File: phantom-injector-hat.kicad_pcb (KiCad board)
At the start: 2 copper layers, 65 x 44.8 mm, 42 parts, among them J1 Conn_02x20_Odd_Even, J2 Conn_02x03_Top_Bottom, J3 Conn_01x03, J4 Conn_01x03, SW1 SW_SPST, U1 LT8362EMSE-PBF

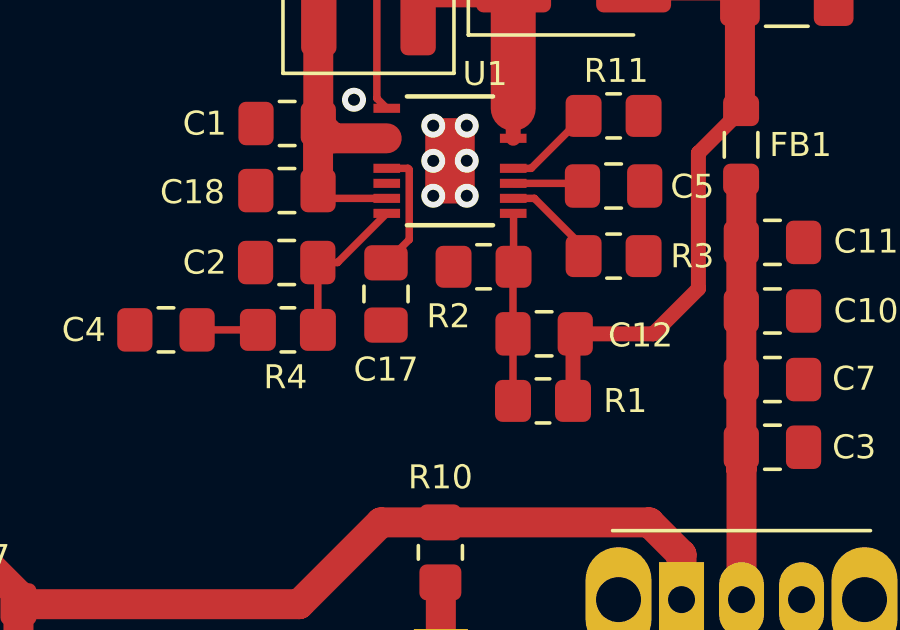
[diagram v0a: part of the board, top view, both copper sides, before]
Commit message: WIP
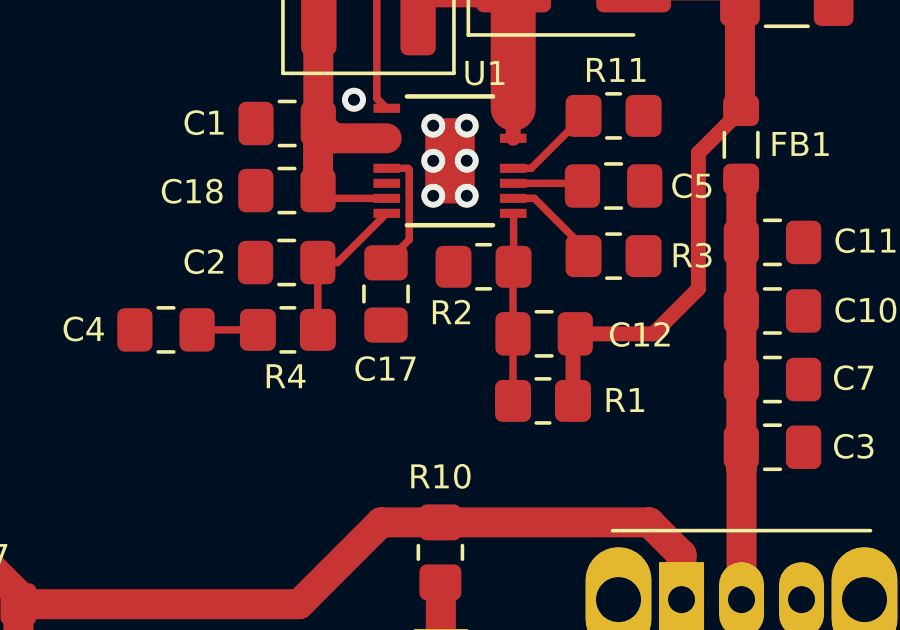
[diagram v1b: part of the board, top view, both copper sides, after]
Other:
- board text removed: "Extend PCB edge 0.5mm if using SMT header"
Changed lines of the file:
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@@
 		(tags "resistor handsolder")
 		(property "Reference" "R2"
-			(at 1.1696 -1.646 180)
+			(at 1.068 -1.5444 180)
 			(layer "F.SilkS")
 			(effects
@@
 		(layer "Edge.Cuts")
 	)
-	(gr_text "Extend PCB edge 0.5mm if using SMT header"
-		(at 103 42.5 0)
-		(layer "Dwgs.User")
-		(effects
-			(font
-				(size 1 1)
-				(thickness 0.15)
-			)
-			(justify left)
-		)
-	)
 	(gr_text "RJ45"
